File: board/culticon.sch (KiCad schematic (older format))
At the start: 78 parts, among them J1 Conn_01x02, J2 Conn_01x02, J3 Conn_01x02, J4 Conn_01x02, J5 Conn_01x04, J6 Conn_01x03, J7 Conn_01x03, J8 Conn_01x03, K1 SANYOU_SRD_Form_C, Q1 BT136-500, Q2 BT136-500, Q3 PN2222A, Q4 PN2222A, SW1 SW_SPST, SW2 SW_SPST, SW3 SW_SPST, T1 Transformer_1P_1S, U1 PC817, U10 RC1602A, U12 24LC64, U13 24LC64, U14 DS1307+, U15 74HC4051, U2 PC817, U3 MOC3021M, U4 MOC3021M, U5 L7805, U6 PC817, U7 PC817, U8 ATmega8-16PU, U9 74HC595, Y1 Crystal

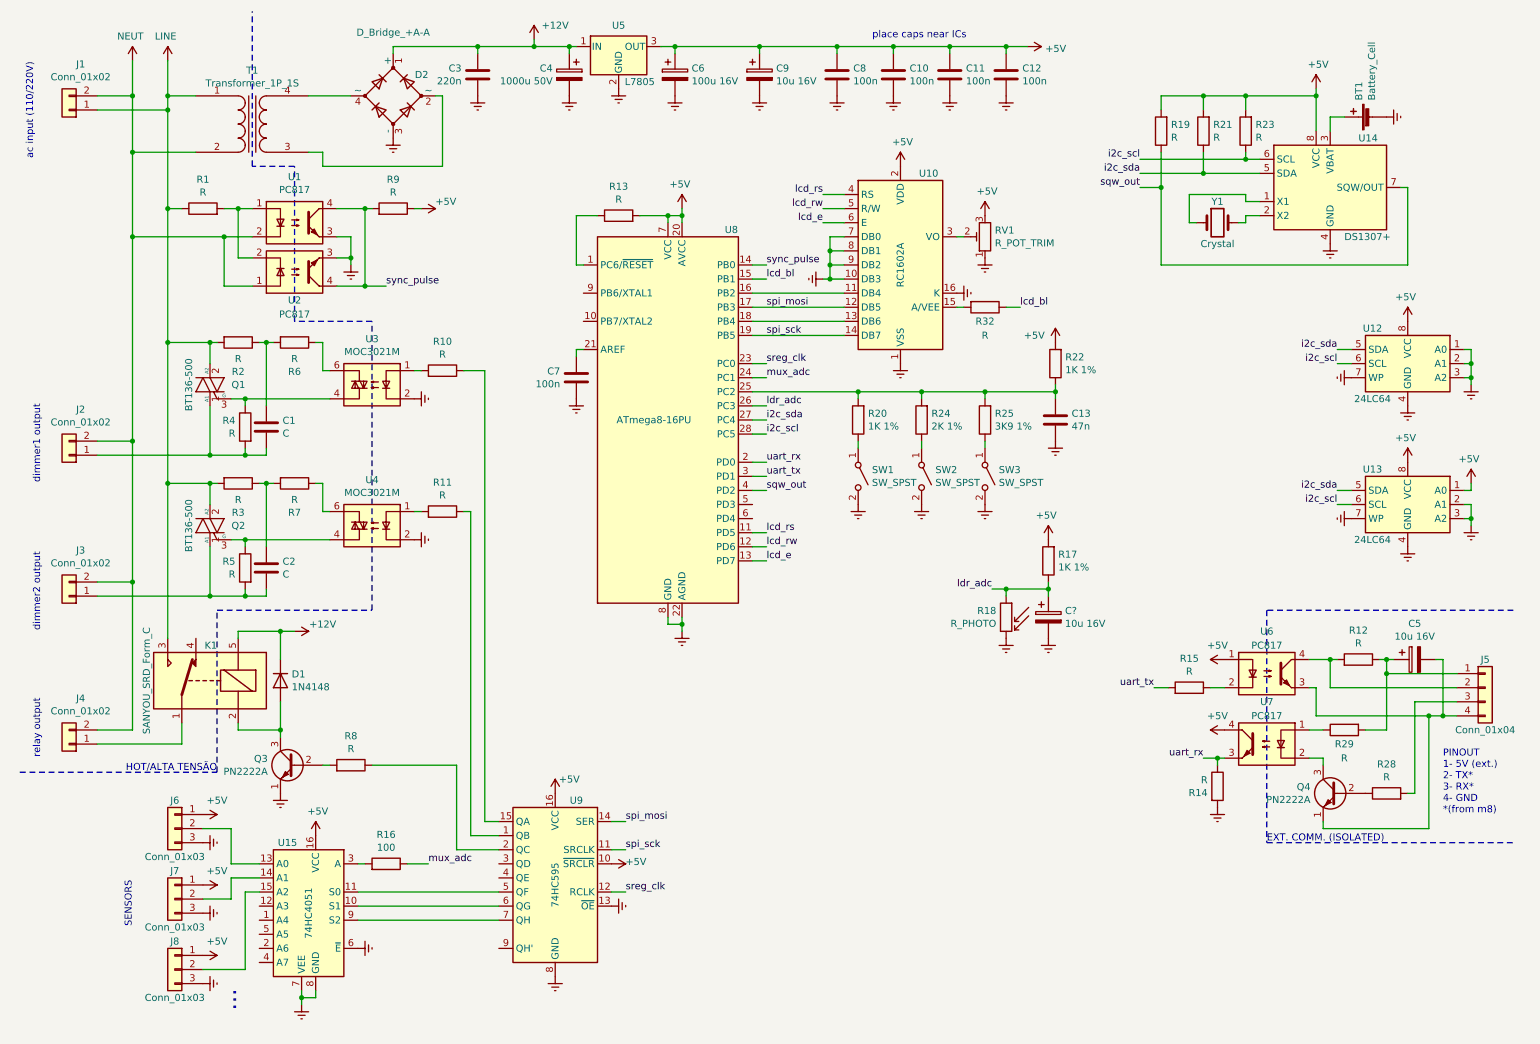
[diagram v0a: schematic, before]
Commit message: board cleanup & optimization
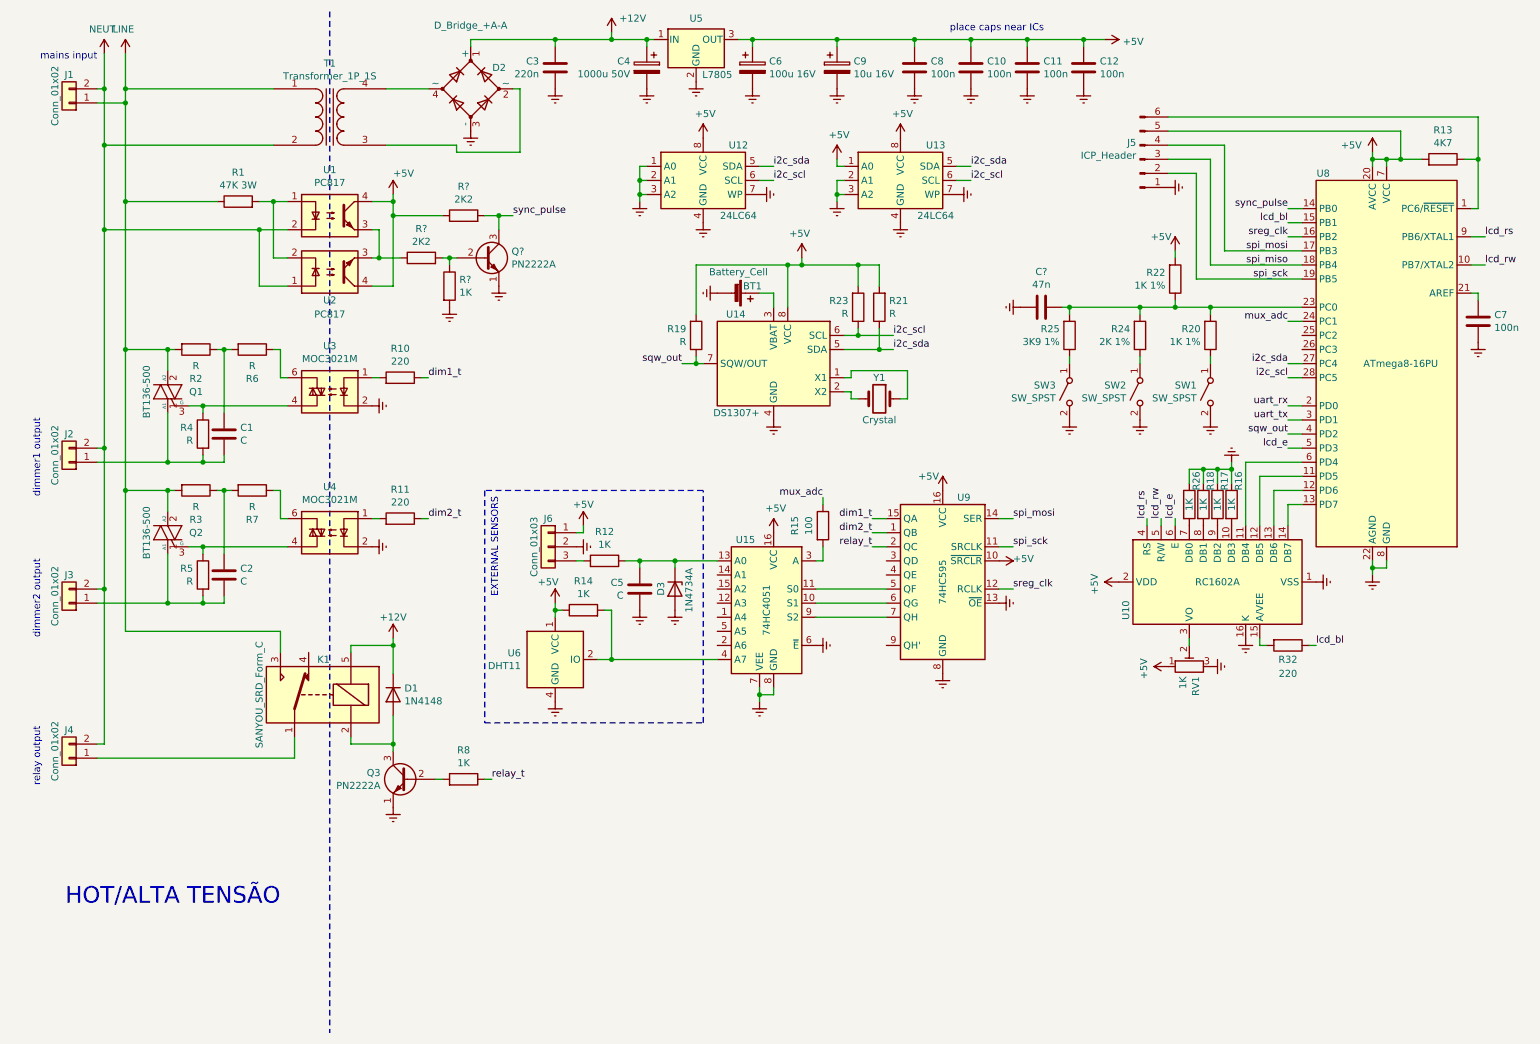
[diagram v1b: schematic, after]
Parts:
- removed C13: 47n, symbol Device:C
- removed C5, C?: 10u 16V, symbol Device:CP
- removed J5: Conn_01x04, symbol Connector_Generic:Conn_01x04
- removed J7, J8: Conn_01x03, symbol Connector_Generic:Conn_01x03
- removed Q4: PN2222A, Package_TO_SOT_THT:TO-92_Inline, symbol Transistor_BJT:PN2222A
- removed R18: R_PHOTO, symbol Device:R_PHOTO
- removed R28, R29, R9: R, symbol Device:R
- removed U6, U7: PC817, Package_DIP:DIP-4_W7.62mm, symbol Isolator:PC817
- added C5: C, symbol Device:C
- added C?: 47n, symbol Device:C
- added D3: 1N4734A, Diode_THT:D_DO-41_SOD81_P10.16mm_Horizontal, symbol Diode:1N47xxA
- added J5: ICP_Header, symbol Connector:Conn_01x06_Male
- added Q?: PN2222A, Package_TO_SOT_THT:TO-92_Inline, symbol Transistor_BJT:PN2222A
- added R18, R26, R?: 1K, symbol Device:R
- added R? (x2): 2K2, symbol Device:R
- added U6: DHT11, Sensor:Aosong_DHT11_5.5x12.0_P2.54mm, symbol Sensor:DHT11
- R1: value R -> 47K 3W
- R10, R11, R32: value R -> 220
- R12, R14, R8: value R -> 1K
- R13: value R -> 4K7
- R15: value R -> 100
- R16: value 100 -> 1K
- R17: value 1K 1% -> 1K
- RV1: value R_POT_TRIM -> 1K
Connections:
- net +5V: now also R14.1, RV1.1, U1.4, U2.4, J5.5 (Pin_5), R?.1, U6.1 (VCC); no longer R17.2, RV1.3
- net Earth: now also J6.2 (Pin_2), R16.1, R17.1, RV1.3, C5.2, C?.1, D3.2 (A), J5.1 (Pin_1), Q?.1 (E), R18.1, R26.1, R?.2, U6.4 (GND); no longer J6.3 (Pin_3), R14.2, RV1.1, U1.3, U10.10 (DB3), U10.7 (DB0), U10.8 (DB1), U10.9 (DB2), U2.3
- net lcd_e: now also U8.5 (PD3); no longer U8.13 (PD7)
- net lcd_rs: now also U8.9 (PB6/XTAL1); no longer U8.11 (PD5)
- net lcd_rw: now also U8.10 (PB7/XTAL2); no longer U8.12 (PD6)
- net mux_adc: now also R15.1; no longer R16.1
- net spi_mosi: now also J5.4 (Pin_4); no longer U10.12 (DB5)
- net spi_sck: now also J5.2 (Pin_2); no longer U10.14 (DB7)
- net sreg_clk: now also U8.16 (PB2); no longer U8.23 (PC0)
- net sync_pulse: now also Q?.3 (C), R?.2; no longer U1.4, U2.4
- net uart_rx: no longer R14.1
- net uart_tx: no longer R15.2
- net relay_t: now reaches R8.1, U9.2 (QC)
- net dim1_t: now reaches R10.1, U9.15 (QA)
- net at R20.2, R22.1, R24.2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: now also U8.23 (PC0), C?.2; no longer U8.25 (PC2)
- net dim2_t: now reaches R11.1, U9.1 (QB)
- net at R13.1, U8.1 (PC6/~RESET): now also J5.6 (Pin_6)
- net at U10.11 (DB4): now also U8.6 (PD4); no longer U8.16 (PB2)
- net at U10.13 (DB6): now also U8.12 (PD6); no longer U8.18 (PB4)
- net at R12.2: now also J6.3 (Pin_3)
- net at R12.1: now also U15.13 (A0), C5.1, D3.1 (K)
- net at R16.2: now also U10.10 (DB3); no longer U15.3 (A)
- net at U15.4 (A7): now also R14.2, U6.2 (IO)
- net ldr_adc: no longer names the net of U8.26 (PC3)
- net ldr_adc: no longer R17.1
- new net: R?.1, U1.3, U2.3
- new net: U10.12 (DB5), U8.11 (PD5)
- new net: U10.14 (DB7), U8.13 (PD7)
- new net: R26.2, U10.7 (DB0)
- new net: R18.2, U10.8 (DB1)
- new net: R17.2, U10.9 (DB2)
- new net: R15.2, U15.3 (A)
- new net: Q?.2 (B), R?.1, R?.2
- new net spi_miso: J5.3 (Pin_3), U8.18 (PB4)
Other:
- note added: "EXTERNAL SENSORS"
- note added: "mains input"
- note removed: "..."
- note removed: "EXT. COMM. (ISOLATED)"
- note removed: "PINOUT\n1- 5V (ext.)\n2- TX*\n3- RX*\n4- GND\n*(from m8)"
- note removed: "SENSORS"
- note removed: "ac input (110/220V)"
- moved on the sheet: C1, C10, C11, C12, C2, C3, C4, C6, C7, C8, C9, D1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
